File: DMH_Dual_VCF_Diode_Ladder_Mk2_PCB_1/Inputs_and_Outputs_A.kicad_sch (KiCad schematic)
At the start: 9 parts, among them J1 TS_Jack_6.35mm_Sw, J2 TS_Jack_6.35mm_Sw, J200 IDC_02x05, J3 TS_Jack_6.35mm_Sw, J4 TS_Jack_6.35mm_Sw, J5 TS_Jack_6.35mm_Sw, J50 Conn_01x06, J60 Conn_01x06, SW8 SW_SPDT_321

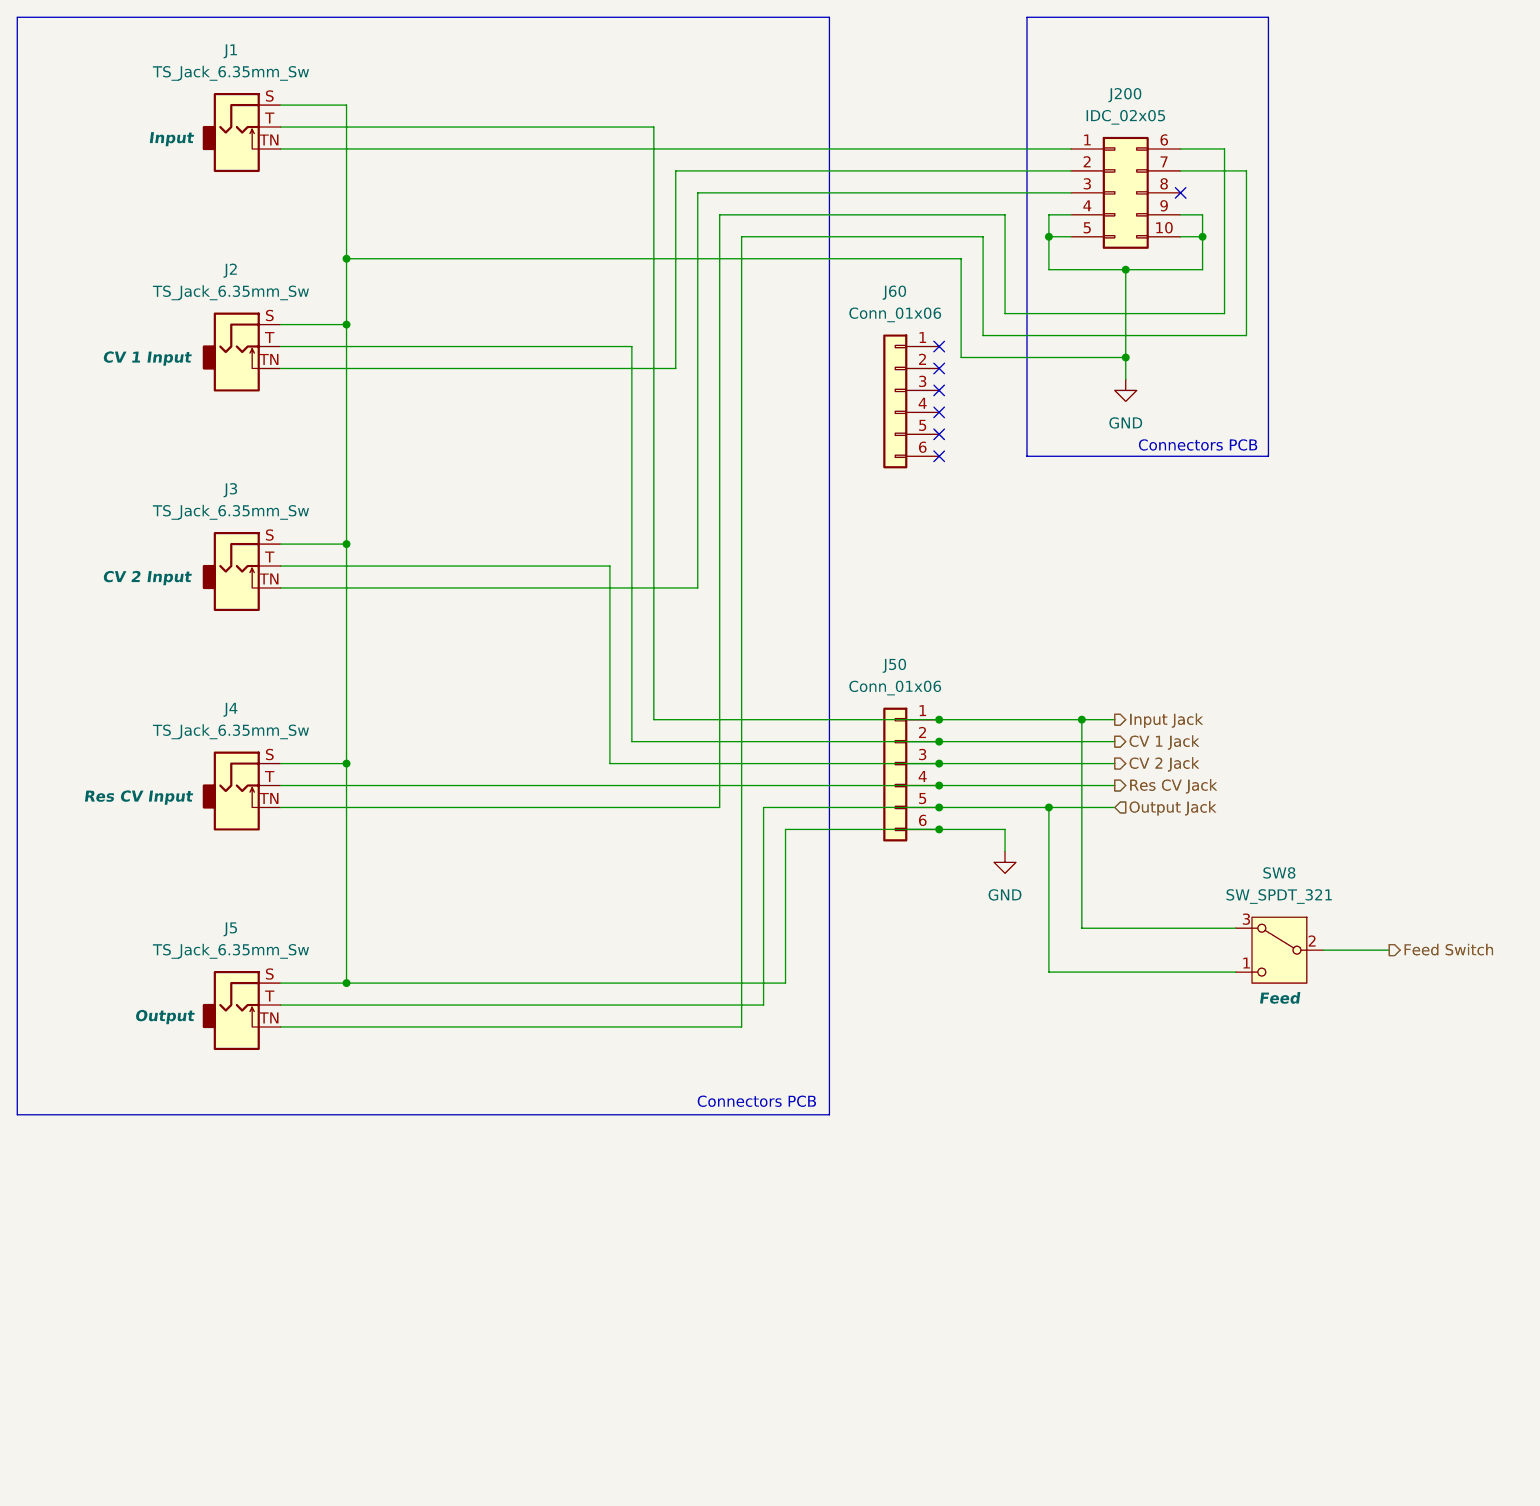
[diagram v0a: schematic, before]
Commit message: Added CV3 and Drive CV to I/O pages
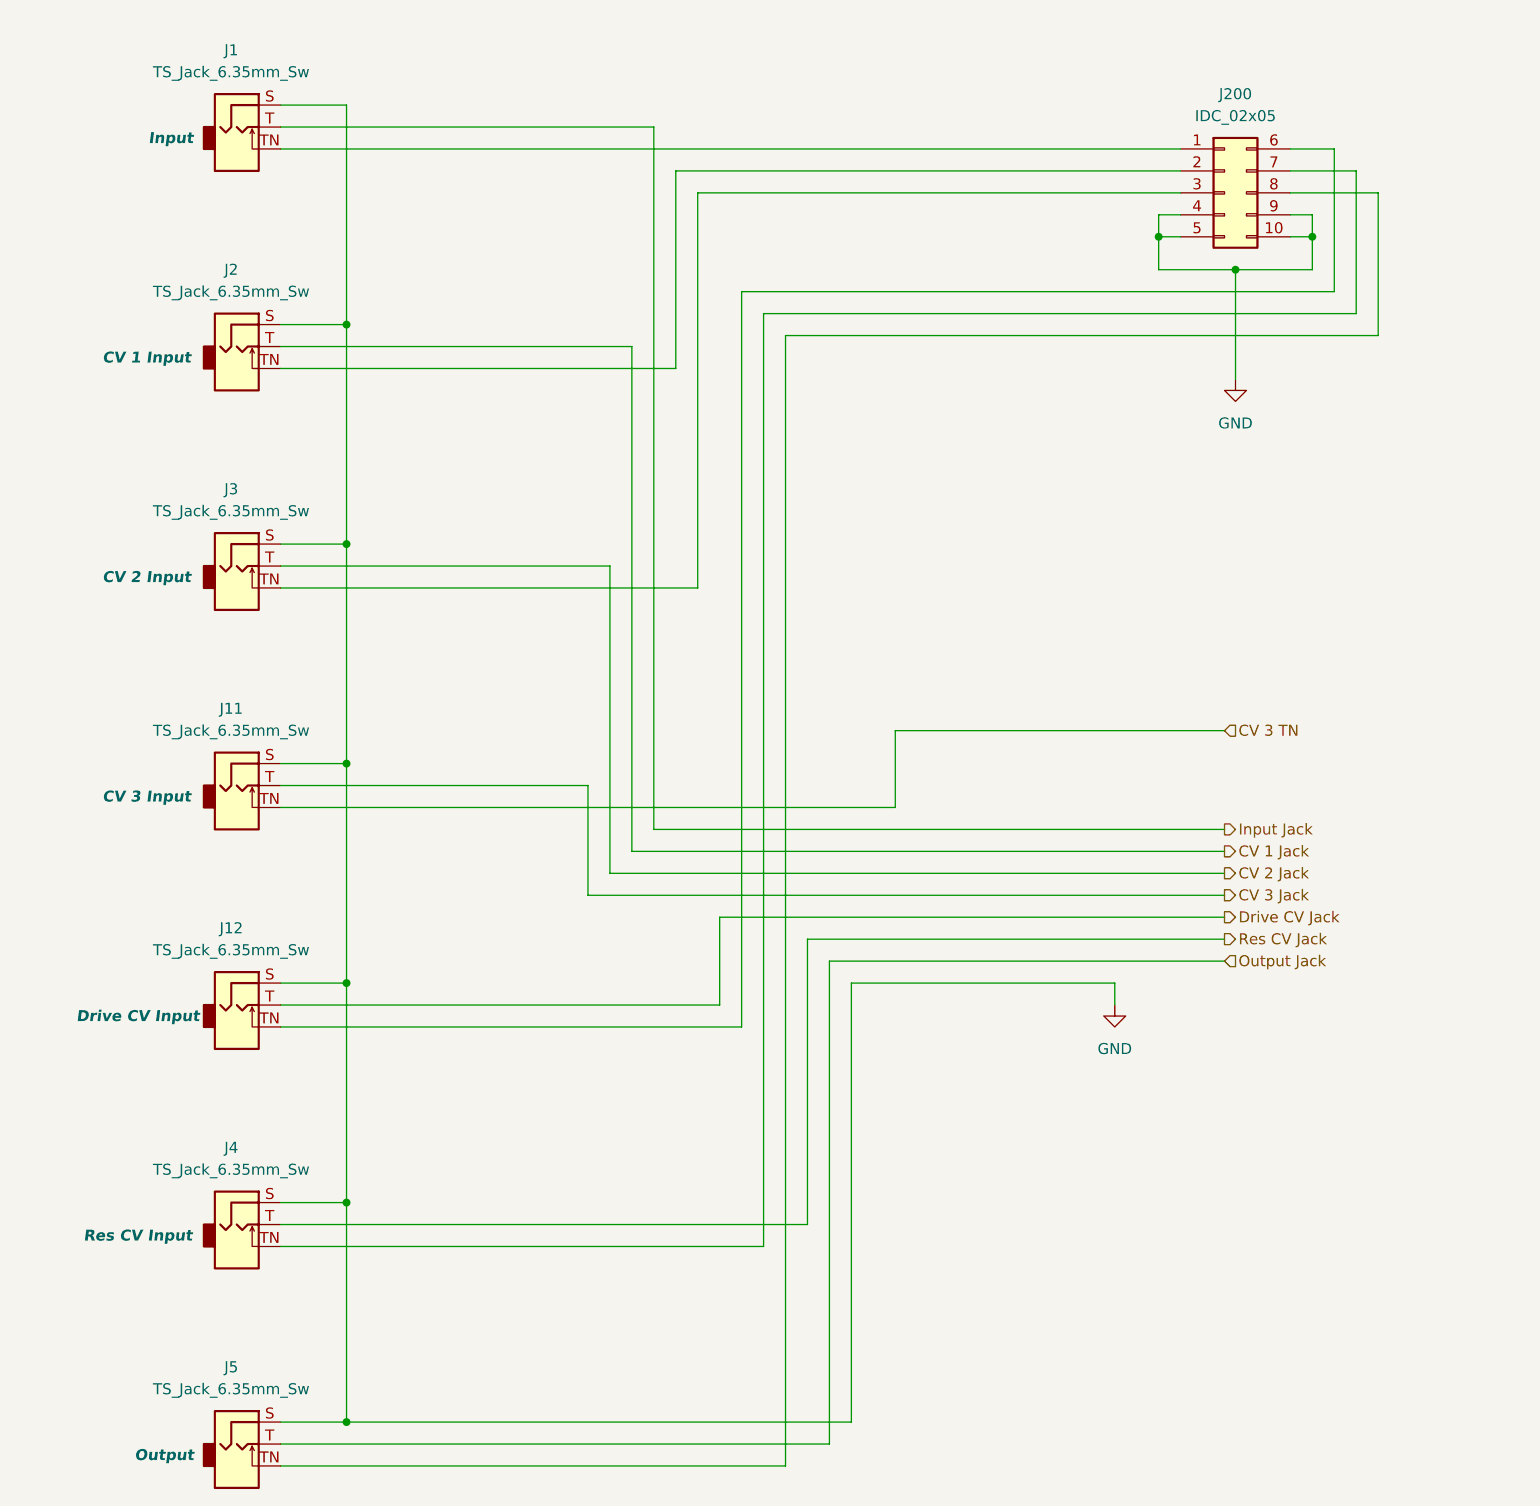
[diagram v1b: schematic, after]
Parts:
- removed J50, J60: Conn_01x06, Connector_PinSocket_2.54mm:PinSocket_1x06_P2.54mm_Vertical, symbol Connector_Generic:Conn_01x06
- removed SW8: SW_SPDT_321, SynthStuff:Toggle_Switch_TE, symbol Switch:SW_SPDT_321
- added J11, J12: TS_Jack_6.35mm_Sw, SynthStuff:CUI_MJ-63052A, symbol SynthStuff:TS_Jack_6.35mm_Sw
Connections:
- net GND: now also J11.S, J12.S
- net at J5.TN: now also J200.8 (Pin_8); no longer J200.7 (Pin_7)
- net at J200.6 (Pin_6): now also J12.TN; no longer J4.TN
- new net: J200.7 (Pin_7), J4.TN
- new net CV 3 Jack: J11.T
- new net CV 3 TN: J11.TN
- new net Drive CV Jack: J12.T
- no-connect marks 7 -> 0
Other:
- note removed: "Connectors PCB"
- moved on the sheet: J200, J4, J5
